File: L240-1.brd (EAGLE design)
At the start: 160 x 100 mm, 16 parts, among them IC1 TINY13-20SSU, IC3 ACS712-LC, K1 G2R2, X4 MKDSN1,5/4-5,08

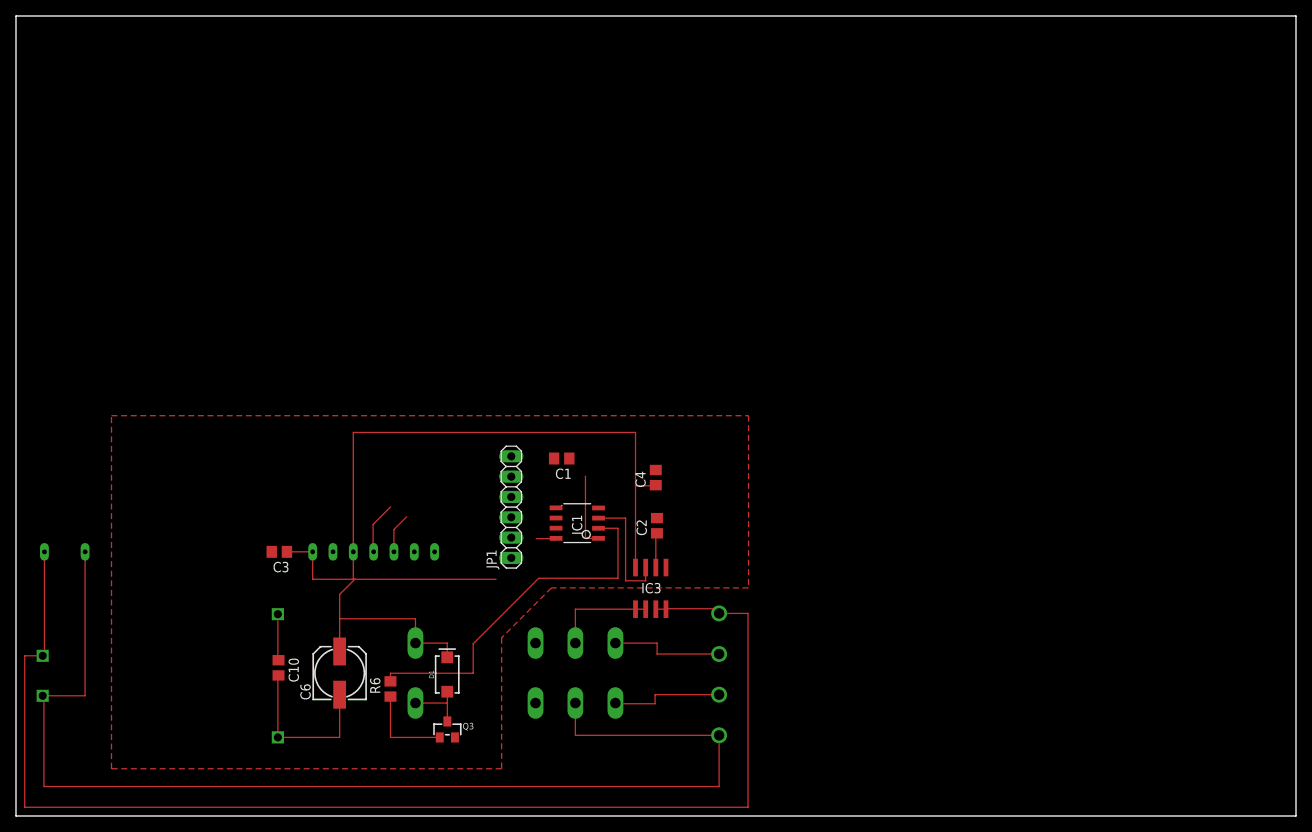
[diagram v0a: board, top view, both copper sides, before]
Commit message: v1.0
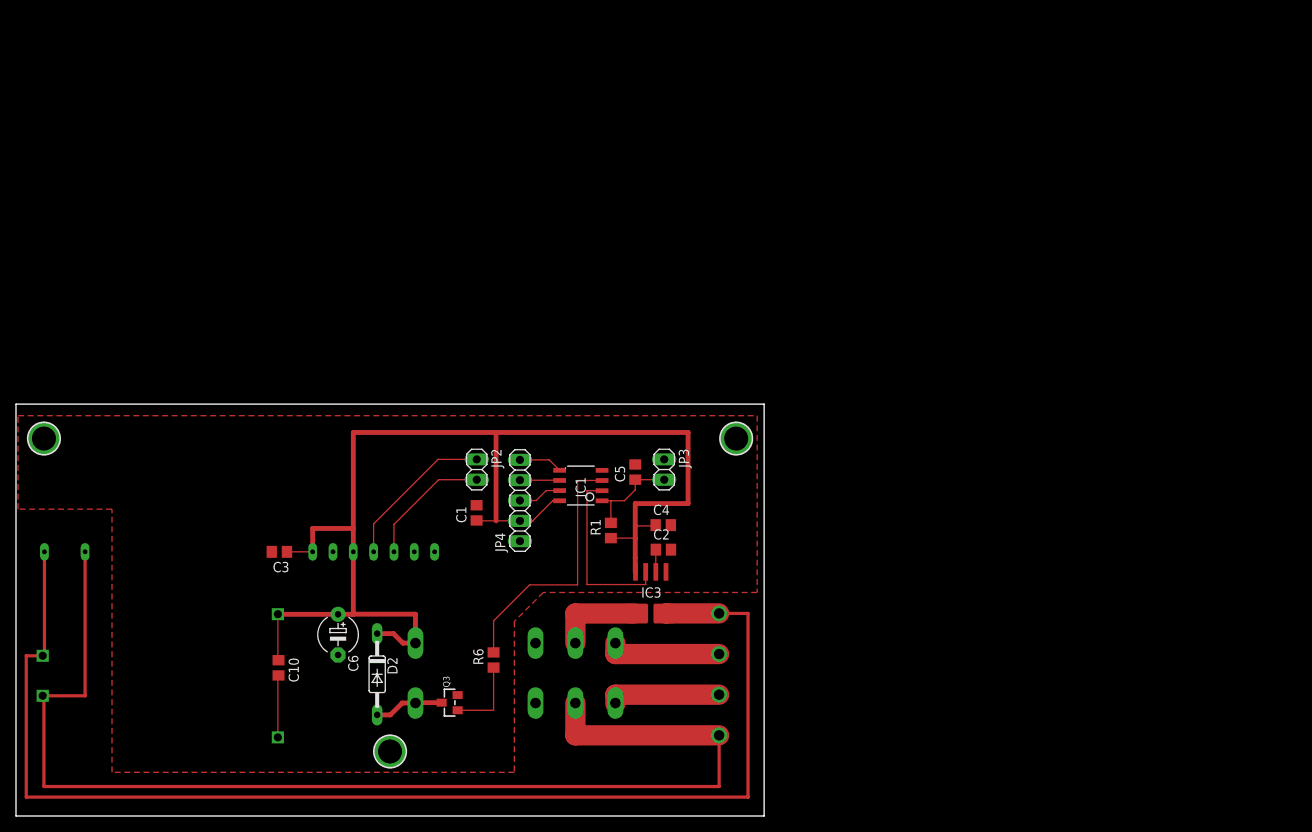
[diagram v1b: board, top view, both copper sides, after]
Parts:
- removed D1: DIODE1N4007, MyLib:SMA-DIODE
- removed JP1: (no value), pinhead:1X06
- added C5: 0.1, rcl:C0805
- added D2: 1N4446, diode:DO35-10
- added JP2, JP3: (no value), pinhead:1X02
- added JP4: (no value), pinhead:1X05
- added R1: 10k, rcl:R0805
- added U$1, U$2, U$3: MOUNTINGHOLE3.0THIN, MyLib:MOUNTINGHOLE_3.0_PLATEDTHIN
- C6: device rcl:153CLV-0605 -> rcl:E5-5
- Q3: value (none) -> BSS138
- moved R6 13.4 mm to (59.7, 19.5)
- moved C1 12.6 mm to (57.6, 37.9), turned to 90 degrees
- moved C4 6.01 mm to (80.9, 36.4), turned to 0 degrees
- moved C6 4.81 mm to (40.3, 22.7), turned to 270 degrees
- moved IC1 4.72 mm to (70.6, 41.3)
- moved Q3 3.36 mm to (54.2, 14.2), turned to 90 degrees
- moved C2 3.10 mm to (80.9, 33.3), turned to 0 degrees
- moved IC3 0.54 mm to (79.3, 27.9)
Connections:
- new net N$1: JP2.1, MD1.RX
- new net N$3: JP2.2, MD1.TX
- net +5V: now also D2.C, JP4.2, R1.1; no longer D1.C, JP1.1
- net GND: now also C5.2, JP3.1, JP4.1; no longer JP1.6
- net LOAD: now also IC1.2; no longer IC1.3
- net MISO: now also JP4.4; no longer JP1.3, MD1.TX
- net MOSI: now also JP4.5; no longer JP1.4, MD1.RX
- net N$13: now also D2.A; no longer D1.A
- net OUT1: now also IC1.3; no longer IC1.2
- net RESET: now also C5.1, JP3.2, R1.2; no longer JP1.5
- net SCK: now also JP4.3; no longer JP1.2
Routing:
- net +5V: track 139.6 -> 160.3 mm
- net N$1: track 0.00 -> 19.7 mm
- net N$3: track 0.00 -> 16.1 mm
- net GND: track 20.8 -> 7.78 mm
- net OUT1: track 45.4 -> 32.5 mm
- net LOAD: track 15.4 -> 22.6 mm
- net SCK: track 0.00 -> 5.47 mm
- net L-IN: track 161.3 -> 157.0 mm
- net RESET: track 9.41 -> 12.4 mm
- net N$7: track 4.38 -> 2.82 mm
- net N$11: track 11.3 -> 9.83 mm
- net MOSI: track 6.56 -> 5.50 mm
- net N$13: track 7.72 -> 8.72 mm
- net N$2: track 13.1 -> 12.6 mm
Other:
- board size 160 x 100 mm -> 93.5 x 51.5 mm
